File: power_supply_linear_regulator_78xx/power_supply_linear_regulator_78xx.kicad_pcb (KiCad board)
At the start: 2 copper layers, 40.5 x 46 mm, 15 parts, among them J1 Conn_01x02_Pin, J2 Conn_01x02_Pin, U3 L7812

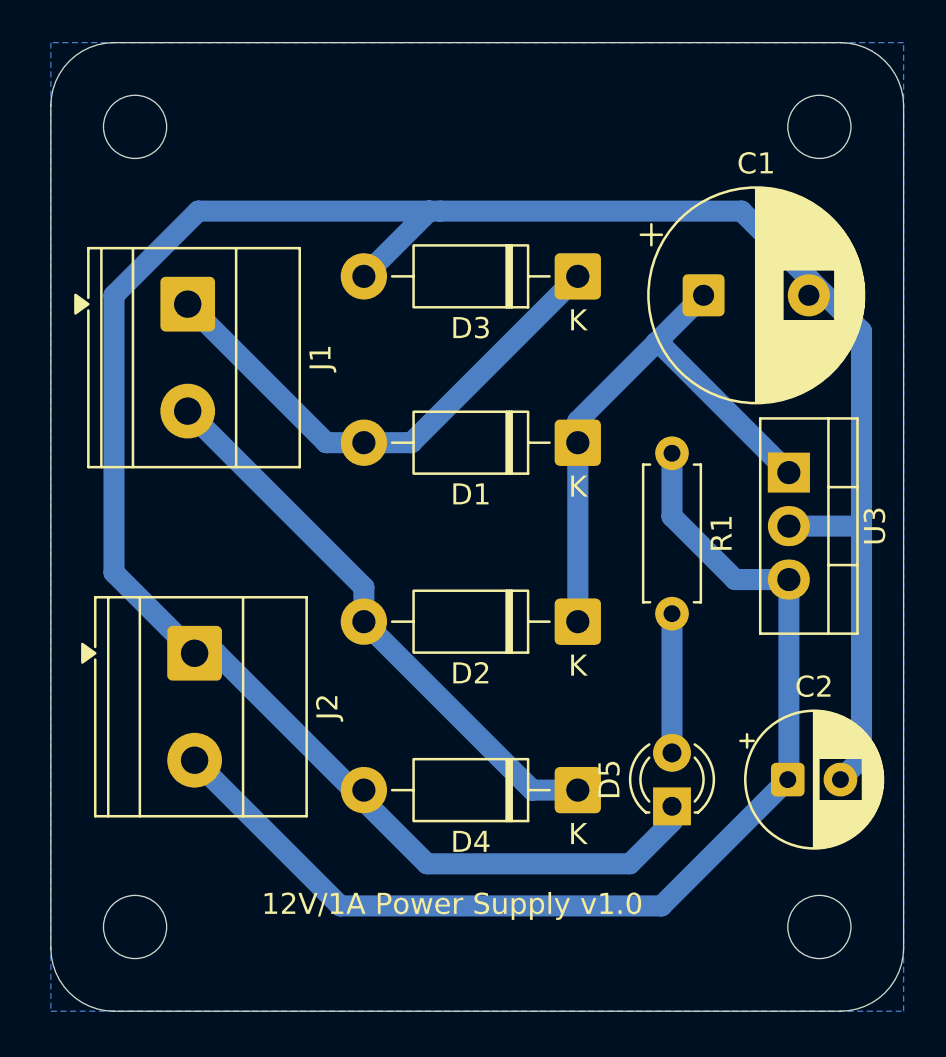
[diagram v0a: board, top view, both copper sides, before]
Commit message: v1.0.0
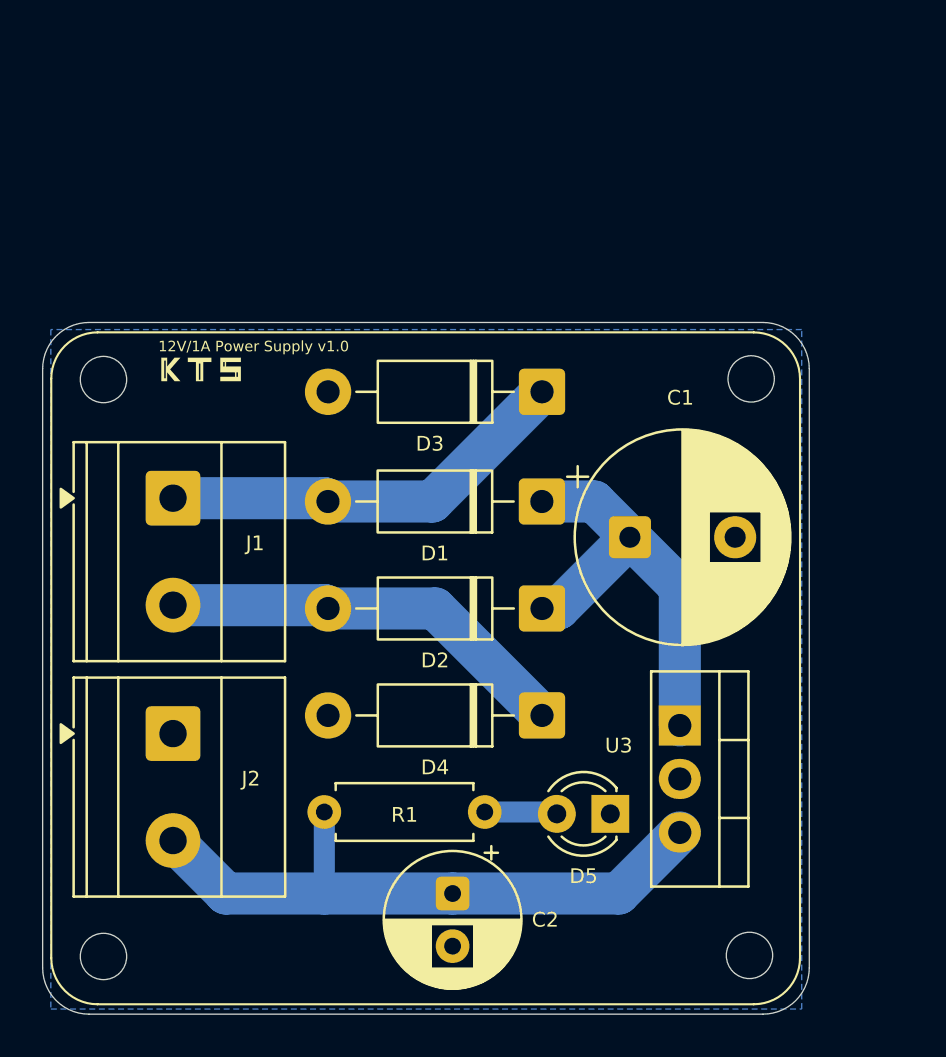
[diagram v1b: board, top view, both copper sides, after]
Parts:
- removed the REF** at (121.0, 55.0)
- removed the REF** at (88.5, 55.0)
- removed the REF** at (121.0, 93.0)
- removed the REF** at (88.5, 93.0)
- added REF**: MountingHole_2.2mm_M2, MountingHole:MountingHole_2.2mm_M2, F.Cu at (87.0, 67.0)
- added REF**: MountingHole_2.2mm_M2, MountingHole:MountingHole_2.2mm_M2, F.Cu at (117.7, 94.3)
- added REF**: MountingHole_2.2mm_M2, MountingHole:MountingHole_2.2mm_M2, F.Cu at (117.8, 67.0)
- added REF**: MountingHole_2.2mm_M2, MountingHole:MountingHole_2.2mm_M2, F.Cu at (87.0, 94.4)
- moved R1 23.7 mm to (97.5, 87.5), turned to 0 degrees
- moved C2 16.8 mm to (103.6, 91.4), turned to -90 degrees
- moved U3 13.1 mm to (114.4, 83.4)
- moved C1 12.0 mm to (112.0, 74.5)
- moved J1 9.24 mm to (90.3, 72.6)
- moved D3 5.74 mm to (107.8, 67.6)
- moved J2 3.95 mm to (90.3, 83.8)
- moved D4 3.93 mm to (107.8, 83.0)
- moved D1 3.27 mm to (107.8, 72.8)
- moved D5 2.95 mm to (111.1, 87.6), turned to 180 degrees
- moved D2 1.81 mm to (107.8, 77.9)
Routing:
- net GND: track 116.0 -> 0.00 mm
- net Net-(J2-Pin_2): track 52.8 -> 30.2 mm
- net Net-(D2-A): track 27.1 -> 19.7 mm
- net Net-(D1-K): track 26.8 -> 20.4 mm
- net Net-(D1-A): track 24.5 -> 19.7 mm
- net Net-(D5-A): track 6.61 -> 3.46 mm
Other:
- board size 40.5 x 46 mm -> 36.4 x 32.8 mm
